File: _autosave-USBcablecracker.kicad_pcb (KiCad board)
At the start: 2 copper layers, 100 x 71 mm, 52 parts, among them IC1 ATTINY85-S, P1 USB_A_L, P10 USB_A_R, P11 USB_B_R, P12 CONN_01X06, P2 USB_B_L, P3 USB_TYPEC-S, P4 USB_MINI_L, P5 USB_MICRO_L, P6 USB_OTG, P7 USB_MINI_R, P8 USB_MICRO_R, P9 USB_TYPEC-S, Q1 S8050, SW1 Switch_SPDT_x2, U1 PCF8574, U2 LMV358, U3 AD623

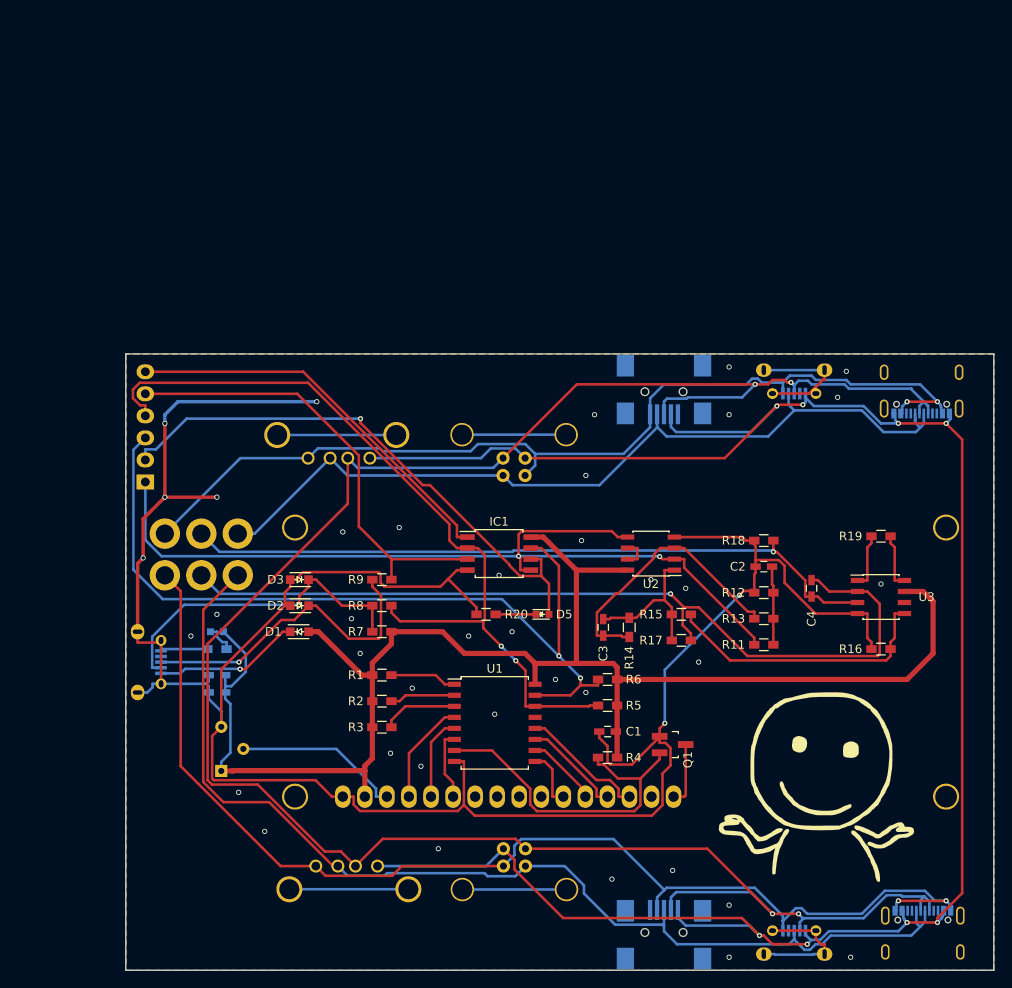
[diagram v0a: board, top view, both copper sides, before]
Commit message: update pcb
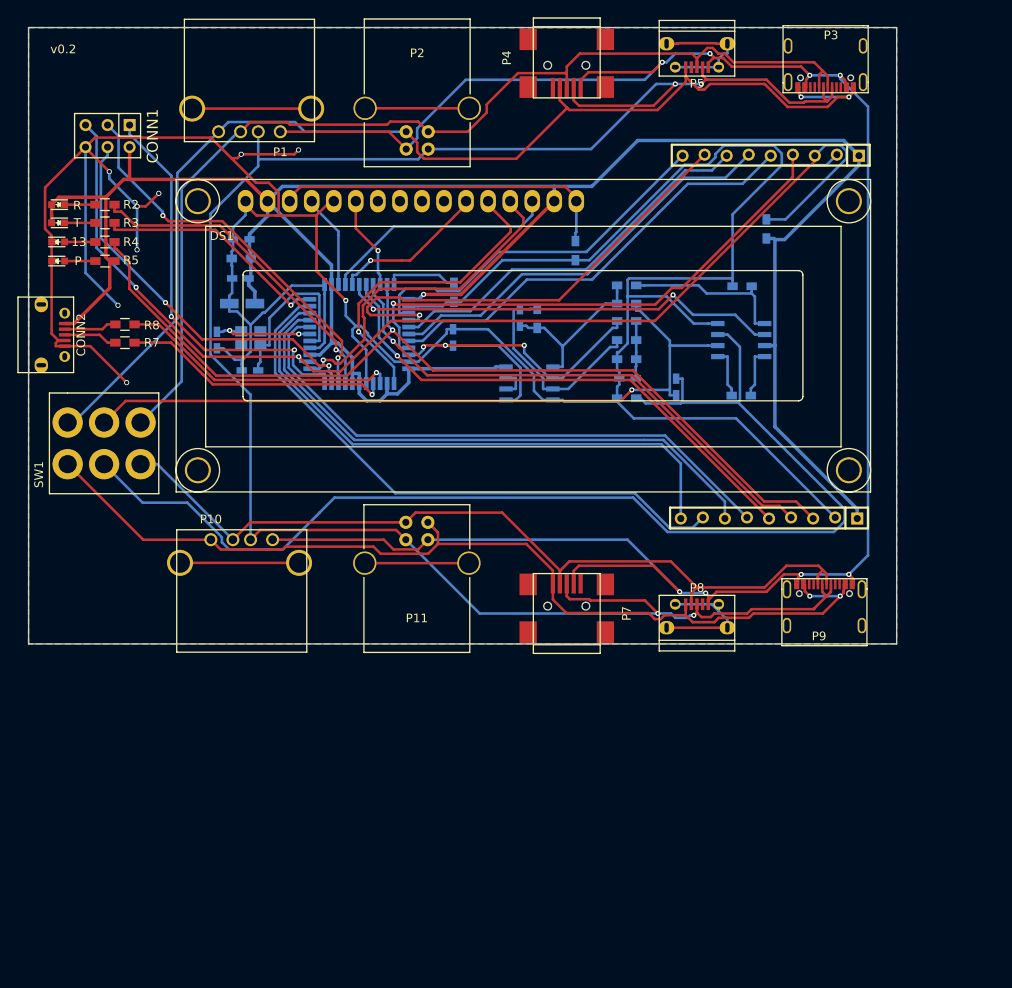
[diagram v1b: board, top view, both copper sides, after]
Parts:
- removed D5: BLUE, LEDs:LED_0603
- removed D6: RED, LEDs:LED_0603
- removed IC1: ATTINY85-S, Housings_SOIC:SOIJ-8_5.3x5.3mm_Pitch1.27mm
- removed Q1: S8050, TO_SOT_Packages_SMD:SOT-23_Handsoldering
- removed R20: 470R, Resistors_SMD:R_0603_HandSoldering
- removed R21: 1K, Resistors_SMD:R_0603_HandSoldering
- removed RV1: POT, USBcablecracker:BOURNS-3362P_pot
- added C7: 1uF, Capacitors_SMD:C_0603_HandSoldering, B.Cu at (74.5, 74.4)
- added C8: 22uF, Capacitors_Tantalum_SMD:Tantalum_Case-A_EIA-3216-18_Wave, B.Cu at (74.6, 81.8)
- added C9: 100nF, Capacitors_SMD:C_0603_HandSoldering, B.Cu at (74.4, 78.9)
- added CONN1: ICSP, Connectors:CONN_2.54mm_2x3, F.Cu at (59.1, 62.5)
- added CONN2: USB_B, SmartEye:USB_Micro-B, F.Cu at (52.6, 85.4)
- added D4: ON, LEDs:LED_0603, F.Cu at (53.4, 76.9)
- added R10: 91R, Resistors_SMD:R_0603_HandSoldering, B.Cu at (113.0, 75.7)
- added Y1: 16MHz, Crystals:crystal_FA238-TSX3225, B.Cu at (75.6, 85.8)
- C1: value 0.1uF -> 22P; moved to B.Cu
- C2, C3, C4, G***, R1, R11, R12, R14, R15, R16, R18, R19, U2, U3: moved to B.Cu
- C5: value 4.7uF -> 22P
- C6: value 0.1uF -> 100nF
- D1: value S4 -> RX; footprint AirBox:SOD-323 -> LEDs:LED_0603
- D2: value W4 -> TX; footprint AirBox:SOD-323 -> LEDs:LED_0603
- D3: value W4 -> L; footprint AirBox:SOD-323 -> LEDs:LED_0603
- DS1, P1, P10, P11, P2, P3, P4, P5, P7, P8, P9, SW1: moved to F.Cu
- P12: value CONN_01X06 -> CONN_01X09; footprint Pin_Headers:Pin_Header_Straight_1x06 -> Connectors:CONN_2.54mm_1x9; moved to F.Cu
- P6: value USB_OTG -> CONN_01X09; footprint SmartEye:USB_Micro-B -> Connectors:CONN_2.54mm_1x9; moved to F.Cu
- R13: value 10K -> 100K; moved to B.Cu
- R17: value 10K -> 100R; moved to B.Cu
- R2, R3, R5: value 10K -> 1K
- R6: value 10K -> 1K; moved to B.Cu
- R7: value 1.5K -> 22R
- R8: value 68R -> 22R
- R9: value 68R -> 10K; moved to B.Cu
- U1: value PCF8574 -> ATmega32U4-AU; footprint Housings_SOIC:SOIC-16W_7.5x10.3mm_Pitch1.27mm -> Housings_QFP:TQFP-44_10x10mm_Pitch0.8mm; moved to B.Cu
- moved P5 103.2 mm to (127.0, 53.0)
- moved P3 102.2 mm to (141.5, 53.5)
- moved P4 102.2 mm to (112.0, 53.5), turned to 270 degrees
- moved P6 92.6 mm to (135.5, 64.7), turned to 0 degrees
- moved P1 85.3 mm to (79.0, 62.0)
- moved R4 83.0 mm to (58.8, 74.7), turned to 0 degrees
- moved P2 81.4 mm to (93.5, 64.0), turned to 90 degrees
- moved R5 77.3 mm to (58.8, 76.9), turned to 0 degrees
- moved P12 72.0 mm to (135.3, 106.5)
- moved DS1 69.5 mm to (75.0, 70.0)
- moved R1 67.9 mm to (135.0, 73.2), turned to 90 degrees
- moved R3 66.3 mm to (58.8, 72.5), turned to 0 degrees
- moved R2 65.5 mm to (58.8, 70.4), turned to 0 degrees
- moved C1 63.7 mm to (71.7, 86.0), turned to 270 degrees
- moved D1 56.5 mm to (53.4, 70.4), turned to 180 degrees
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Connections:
- C1 pad 1: +5V -> Net-(C1-Pad1)
- C5 pad 1: +5V -> Net-(C5-Pad1)
- C6 pad 1: +5V -> /AREF
- D1 pad 2: +5V -> +5C
- D2 pad 2: GND -> +5C
- D3 pad 1: Net-(D3-Pad1) -> GND
- D3 pad 2: GND -> Net-(D3-Pad2)
- DS1 pad 11: /DB4 -> /D6
- DS1 pad 12: /DB5 -> /D7
- DS1 pad 13: /DB6 -> /IO11
- DS1 pad 14: /DB7 -> /IO12
- DS1 pad 15: /A -> +5C
- DS1 pad 16: /K -> Net-(DS1-Pad16)
- DS1 pad 2: +5V -> +5C
- DS1 pad 3: /VO -> Net-(DS1-Pad16)
- DS1 pad 4: /RS -> /D4
- DS1 pad 5: /RW -> GND
- DS1 pad 6: /CS -> /D5
- P12 pad 1: /AREF -> +5C
- P12 pad 2: Net-(D5-Pad2) -> GND
- P12 pad 3: /SDA -> /IO13
- P12 pad 4: /SCL -> /IO10
- P12 pad 5: Net-(IC1-Pad3) -> /IO9
- P12 pad 6: Net-(IC1-Pad1) -> /D3
- P6 pad 1: Net-(D1-Pad1) -> +5C
- P6 pad 2: Net-(D3-Pad1) -> GND
- P6 pad 3: Net-(D2-Pad1) -> /RESET
- P6 pad 4: Net-(P6-Pad4) -> /A5
- P6 pad 5: GND -> /A4
- P6 pad 6: GND -> /A3
- R1 pad 1: Net-(R1-Pad1) -> +5C
- R1 pad 2: +5V -> /RESET
- R2 pad 1: Net-(R2-Pad1) -> Net-(D1-Pad1)
- R2 pad 2: +5V -> /RX_LED
- R3 pad 1: Net-(R3-Pad1) -> Net-(D2-Pad1)
- R3 pad 2: +5V -> /TX_LED
- R4 pad 1: +5V -> Net-(D3-Pad2)
- R4 pad 2: /P3 -> /IO13
- R5 pad 1: +5V -> Net-(D4-Pad2)
- R5 pad 2: /SCL -> +5C
- R6 pad 1: +5V -> GND
- R6 pad 2: /SDA -> /HWB
- R7 pad 1: +5V -> /D+
- R7 pad 2: Net-(D3-Pad1) -> Net-(CONN2-Pad3)
- R8 pad 1: /SCL -> /D-
- R8 pad 2: Net-(D3-Pad1) -> Net-(CONN2-Pad2)
- R9 pad 1: Net-(IC1-Pad3) -> GND
- R9 pad 2: Net-(D2-Pad1) -> +5C
- U1 pad 1: Net-(R1-Pad1) -> /D7
- U1 pad 10: /DB5 -> /MOSI
- U1 pad 11: /DB6 -> /MISO
- U1 pad 12: /DB7 -> /IO11
- U1 pad 13: Net-(U1-Pad13) -> /RESET
- U1 pad 14: /SCL -> +5C
- U1 pad 15: /SDA -> GND
- U1 pad 16: +5V -> Net-(C5-Pad1)
- U1 pad 2: Net-(R2-Pad1) -> +5C
- U1 pad 3: Net-(R3-Pad1) -> /D-
- U1 pad 4: /RS -> /D+
- U1 pad 5: /RW -> GND
- U1 pad 6: /CS -> +5C
- U1 pad 7: /P3 -> +5C
- U1 pad 8: GND -> /RX_LED
- U1 pad 9: /DB4 -> /SCK
- U2 pad 8: +5V -> +5C
- U3 pad 6: /TO_ADC -> /IO8
- U3 pad 7: +5V -> +5C
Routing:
- net +5C: track 0.00 -> 264.7 mm, vias 0 -> 1
- net +5V: track 178.3 -> 0.00 mm
- net /RESET: track 0.00 -> 133.2 mm, vias 0 -> 2
- net /IO13: track 0.00 -> 105.8 mm, vias 0 -> 1
- net /SDA: track 96.2 -> 0.00 mm, vias 2 -> 0
- net GND: track 277.2 -> 371.5 mm, vias 7 -> 9
- net /SCL: track 93.9 -> 0.00 mm, vias 2 -> 0
- net /D1: track 0.00 -> 67.2 mm
- net /D2: track 0.00 -> 66.7 mm
- net /D3: track 0.00 -> 66.5 mm
- net /D0: track 0.00 -> 65.8 mm
- net Net-(D5-Pad2): track 64.1 -> 0.00 mm, vias 1 -> 0
- net /IO10: track 0.00 -> 61.7 mm, vias 0 -> 1
- net /A5: track 0.00 -> 61.3 mm, vias 0 -> 1
- net /IO9: track 0.00 -> 60.3 mm, vias 0 -> 1
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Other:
- net class Default: trace_width 0.4 -> 0.3
- net class power added: clearance 0.2, trace_width 0.4, via_dia 0.6, via_drill 0.4
- board text added: "13"
- board text added: "P"
- board text added: "R"
- board text added: "T"
- board text added: "v0.2"
- board text removed: "SCL"
- board text removed: "SDA"
- board text removed: "v0.1"
